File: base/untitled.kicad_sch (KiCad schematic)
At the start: 56 parts, among them U23 6N137, U24 6N137, U25 6N137, U26 6N137, U27 6N137, U28 6N137, U29 6N137, U30 6N137, U31 6N137, U32 6N137, U33 6N137, U34 6N137, U36 6N137, U37 6N137

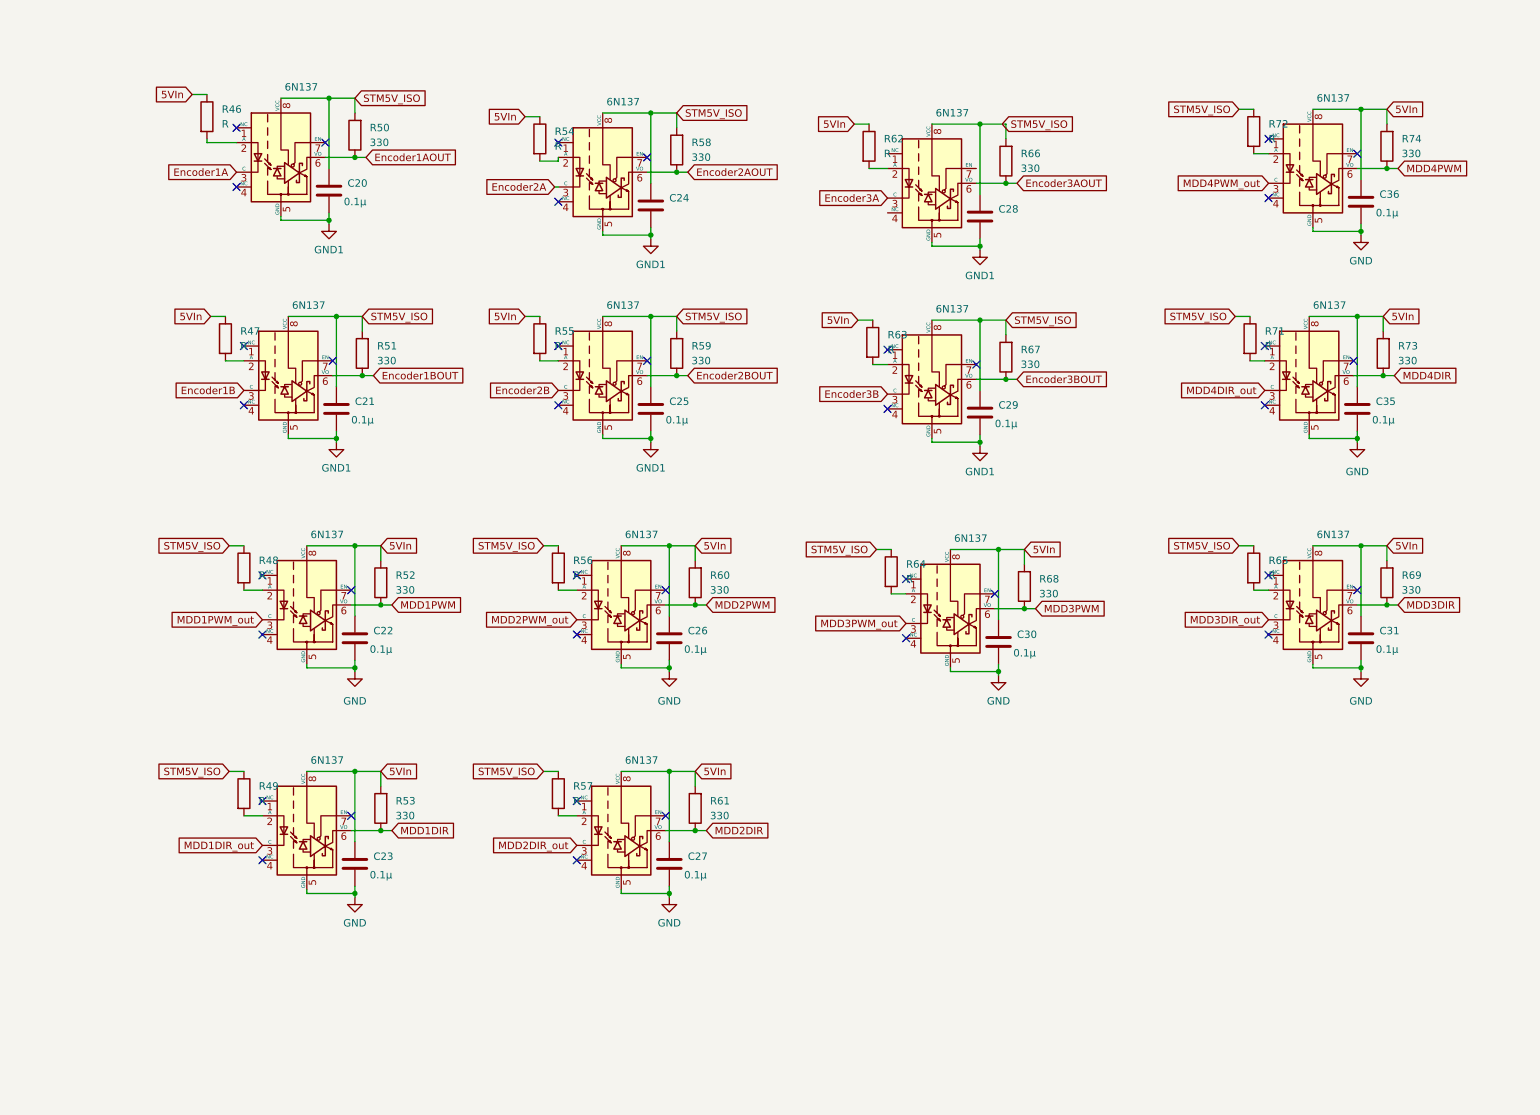
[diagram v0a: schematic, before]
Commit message: changes to schematic
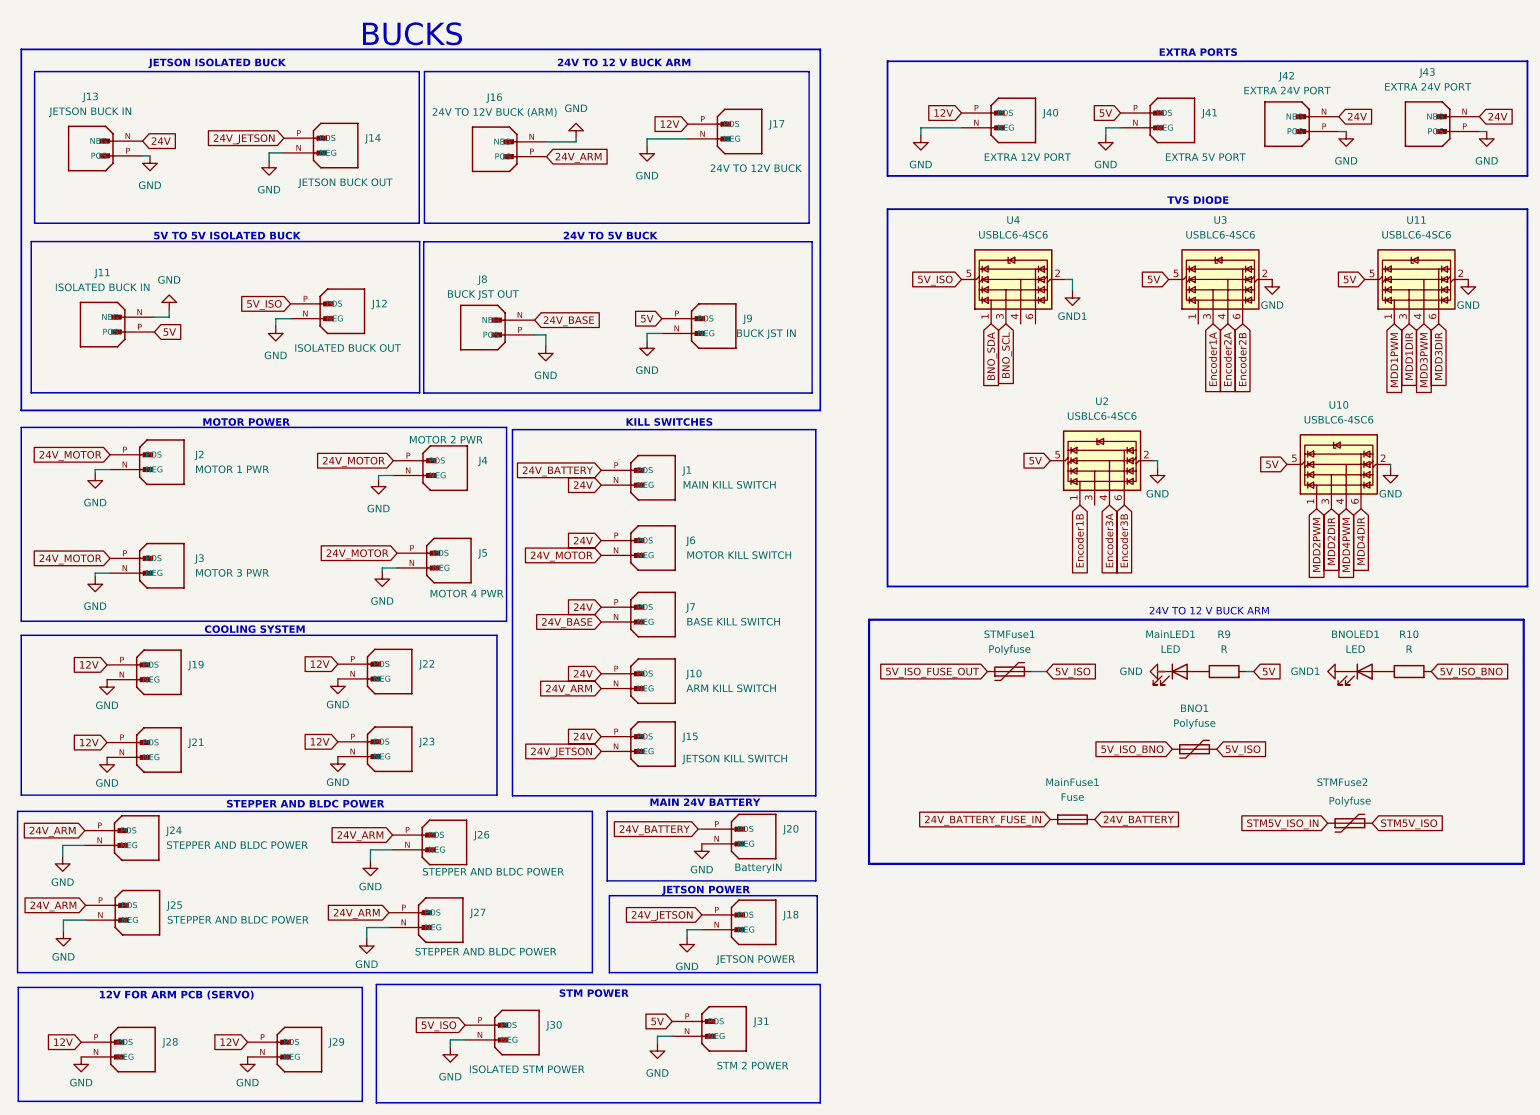
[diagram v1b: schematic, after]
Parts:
- removed C20, C21, C22, C23, C24, C25, C26, C27, C28, C29, C30, C31, C35, C36: 0.1µ, symbol Device:C
- removed R46, R47, R48, R49, R54, R55, R56, R57, R62, R63, R64, R65, R71, R72: R, symbol Device:R
- removed R50, R51, R52, R53, R58, R59, R60, R61, R66, R67, R68, R69, R73, R74: 330, symbol Device:R
- removed U23, U24, U25, U26, U27, U28, U29, U30, U31, U32, U33, U34, U36, U37: 6N137, Package_DIP:DIP-8_W7.62mm, symbol Isolator:6N137
- added BNO1, STMFuse1, STMFuse2: Polyfuse, Fuse:Fuse_0603_1608Metric_Pad1.05x0.95mm_HandSolder, symbol Device:Polyfuse
- added BNOLED1, MainLED1: LED, LED_SMD:LED_0201_0603Metric, symbol Device:LED
- added J1: MAIN KILL SWITCH, Connector_AMASS:AMASS_XT60-M_1x02_P7.20mm_Vertical, symbol XT60-M:XT60-M
- added J10: ARM KILL SWITCH, Connector_AMASS:AMASS_XT60-M_1x02_P7.20mm_Vertical, symbol XT60-M:XT60-M
- added J11: ISOLATED BUCK IN, Connector_AMASS:AMASS_XT60-M_1x02_P7.20mm_Vertical, symbol XT60-M:XT60-M
- added J12: ISOLATED BUCK OUT, Connector_AMASS:AMASS_XT60-M_1x02_P7.20mm_Vertical, symbol XT60-M:XT60-M
- added J13: JETSON BUCK IN, Connector_AMASS:AMASS_XT60-M_1x02_P7.20mm_Vertical, symbol XT60-M:XT60-M
- added J14: JETSON BUCK OUT, Connector_AMASS:AMASS_XT60-M_1x02_P7.20mm_Vertical, symbol XT60-M:XT60-M
- added J15: JETSON KILL SWITCH, Connector_AMASS:AMASS_XT60-M_1x02_P7.20mm_Vertical, symbol XT60-M:XT60-M
- added J16: 24V TO 12V BUCK (ARM), Connector_AMASS:AMASS_XT60-M_1x02_P7.20mm_Vertical, symbol XT60-M:XT60-M
- added J17: 24V TO 12V BUCK, Connector_AMASS:AMASS_XT60-M_1x02_P7.20mm_Vertical, symbol XT60-M:XT60-M
- added J18: JETSON POWER, Connector_AMASS:AMASS_XT60-M_1x02_P7.20mm_Vertical, symbol XT60-M:XT60-M
- added J19, J21, J22, J23, J28, J29: 12V_BUCK_PINOUTS_ARM, Connector_AMASS:AMASS_XT60-M_1x02_P7.20mm_Vertical, symbol XT60-M:XT60-M
- added J2: MOTOR 1 PWR, Connector_AMASS:AMASS_XT60-M_1x02_P7.20mm_Vertical, symbol XT60-M:XT60-M
- added J20: BatteryIN, Connector_AMASS:AMASS_XT60-M_1x02_P7.20mm_Vertical, symbol XT60-M:XT60-M
- added J24, J25, J26, J27: STEPPER AND BLDC POWER, Connector_AMASS:AMASS_XT60-M_1x02_P7.20mm_Vertical, symbol XT60-M:XT60-M
- added J3: MOTOR 3 PWR, Connector_AMASS:AMASS_XT60-M_1x02_P7.20mm_Vertical, symbol XT60-M:XT60-M
- added J30: ISOLATED STM POWER, Connector_AMASS:AMASS_XT60-M_1x02_P7.20mm_Vertical, symbol XT60-M:XT60-M
- added J31: STM 2 POWER, Connector_AMASS:AMASS_XT60-M_1x02_P7.20mm_Vertical, symbol XT60-M:XT60-M
- added J4: MOTOR 2 PWR, Connector_AMASS:AMASS_XT60-M_1x02_P7.20mm_Vertical, symbol XT60-M:XT60-M
- added J40: EXTRA 12V PORT, Connector_AMASS:AMASS_XT60-M_1x02_P7.20mm_Vertical, symbol XT60-M:XT60-M
- added J41: EXTRA 5V PORT, Connector_AMASS:AMASS_XT60-M_1x02_P7.20mm_Vertical, symbol XT60-M:XT60-M
- added J42, J43: EXTRA 24V PORT, Connector_AMASS:AMASS_XT60-M_1x02_P7.20mm_Vertical, symbol XT60-M:XT60-M
- added J5: MOTOR 4 PWR, Connector_AMASS:AMASS_XT60-M_1x02_P7.20mm_Vertical, symbol XT60-M:XT60-M
- added J6: MOTOR KILL SWITCH, Connector_AMASS:AMASS_XT60-M_1x02_P7.20mm_Vertical, symbol XT60-M:XT60-M
- added J7: BASE KILL SWITCH, Connector_AMASS:AMASS_XT60-M_1x02_P7.20mm_Vertical, symbol XT60-M:XT60-M
- added J8: BUCK JST OUT, Connector_AMASS:AMASS_XT60-M_1x02_P7.20mm_Vertical, symbol XT60-M:XT60-M
- added J9: BUCK JST IN, Connector_AMASS:AMASS_XT60-M_1x02_P7.20mm_Vertical, symbol XT60-M:XT60-M
- added MainFuse1: Fuse, Fuse:Fuseholder_Littelfuse_445_030_series_5x30mm, symbol Device:Fuse
- added R10, R9: R, PCM_4ms_Resistor:R_0603, symbol Device:R
- added U10, U11, U2, U3, U4: USBLC6-4SC6, Package_TO_SOT_SMD:SOT-23-6, symbol Power_Protection:USBLC6-4SC6
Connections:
- net Encoder1A: now also U3.3 (I/O2)
- net Encoder1B: now also U2.1 (I/O1)
- net Encoder2A: now also U3.4 (I/O3)
- net Encoder2B: now also U3.6 (I/O4)
- net Encoder3A: now also U2.4 (I/O3)
- net Encoder3B: now also U2.6 (I/O4)
- net GND: now also J11.N (NEG), J12.N (NEG), J13.P (POS), J14.N (NEG), J16.N (NEG), J17.N (NEG), J18.N (NEG), J19.N (NEG), J2.N (NEG), J20.N (NEG), J21.N (NEG), J22.N (NEG), J23.N (NEG), J24.N (NEG), J25.N (NEG), J26.N (NEG), J27.N (NEG), J28.N (NEG), J29.N (NEG), J3.N (NEG), J30.N (NEG), J31.N (NEG), J4.N (NEG), J40.N (NEG), J41.N (NEG), J42.P (POS), J43.P (POS), J5.N (NEG), J8.P (POS), J9.N (NEG), MainLED1.1 (K), U10.2 (GND), U11.2 (GND), U2.2 (GND), U3.2 (GND)
- net GND1: now also BNOLED1.1 (K), U4.2 (GND)
- net MDD1DIR: now also U11.3 (I/O2)
- net MDD1PWM: now also U11.1 (I/O1)
- net MDD2DIR: now also U10.3 (I/O2)
- net MDD2PWM: now also U10.1 (I/O1)
- net MDD3DIR: now also U11.6 (I/O4)
- net MDD3PWM: now also U11.4 (I/O3)
- net MDD4DIR: now also U10.6 (I/O4)
- net MDD4PWM: now also U10.4 (I/O3)
- net STM5V_ISO: now also STMFuse2.2
- new net: BNOLED1.2 (A), R10.1
- new net: MainLED1.2 (A), R9.1
- new net 12V: J17.P (POS), J19.P (POS), J21.P (POS), J22.P (POS), J23.P (POS), J28.P (POS), J29.P (POS), J40.P (POS)
- new net 24V: J1.N (NEG), J10.P (POS), J13.N (NEG), J15.P (POS), J42.N (NEG), J43.N (NEG), J6.P (POS), J7.P (POS)
- new net 24V_ARM: J10.N (NEG), J16.P (POS), J24.P (POS), J25.P (POS), J26.P (POS), J27.P (POS)
- new net 24V_BASE: J7.N (NEG), J8.N (NEG)
- new net 24V_BATTERY: J1.P (POS), J20.P (POS), MainFuse1.1
- new net 24V_BATTERY_FUSE_IN: MainFuse1.2
- new net 24V_JETSON: J14.P (POS), J15.N (NEG), J18.P (POS)
- new net 24V_MOTOR: J2.P (POS), J3.P (POS), J4.P (POS), J5.P (POS), J6.N (NEG)
- new net 5V: J11.P (POS), J31.P (POS), J41.P (POS), J9.P (POS), R9.2, U10.5 (VBUS), U11.5 (VBUS), U2.5 (VBUS), U3.5 (VBUS)
- new net 5V_ISO: BNO1.2, J12.P (POS), J30.P (POS), STMFuse1.2, U4.5 (VBUS)
- new net 5V_ISO_BNO: BNO1.1, R10.2
- new net 5V_ISO_FUSE_OUT: STMFuse1.1
- new net BNO_SCL: U4.3 (I/O2)
- new net BNO_SDA: U4.1 (I/O1)
- new net STM5V_ISO_IN: STMFuse2.1
- no-connect marks 39 -> 0
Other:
- note added: "12V FOR ARM PCB (SERVO)"
- note added: "24V TO 12 V BUCK ARM"
- note added: "24V TO 5V BUCK"
- note added: "5V TO 5V ISOLATED BUCK"
- note added: "BUCKS"
- note added: "COOLING SYSTEM"
- note added: "EXTRA PORTS"
- note added: "JETSON ISOLATED BUCK"
- note added: "JETSON POWER"
- note added: "KILL SWITCHES"
- note added: "MAIN 24V BATTERY"
- note added: "MOTOR POWER"
- note added: "STEPPER AND BLDC POWER"
- note added: "STM POWER"
- note added: "TVS DIODE"
